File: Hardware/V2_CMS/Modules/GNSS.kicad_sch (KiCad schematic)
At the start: 20 parts, among them J3 132134, Q1 SI2302, U3 NEO-M8M, U4 AS193-73

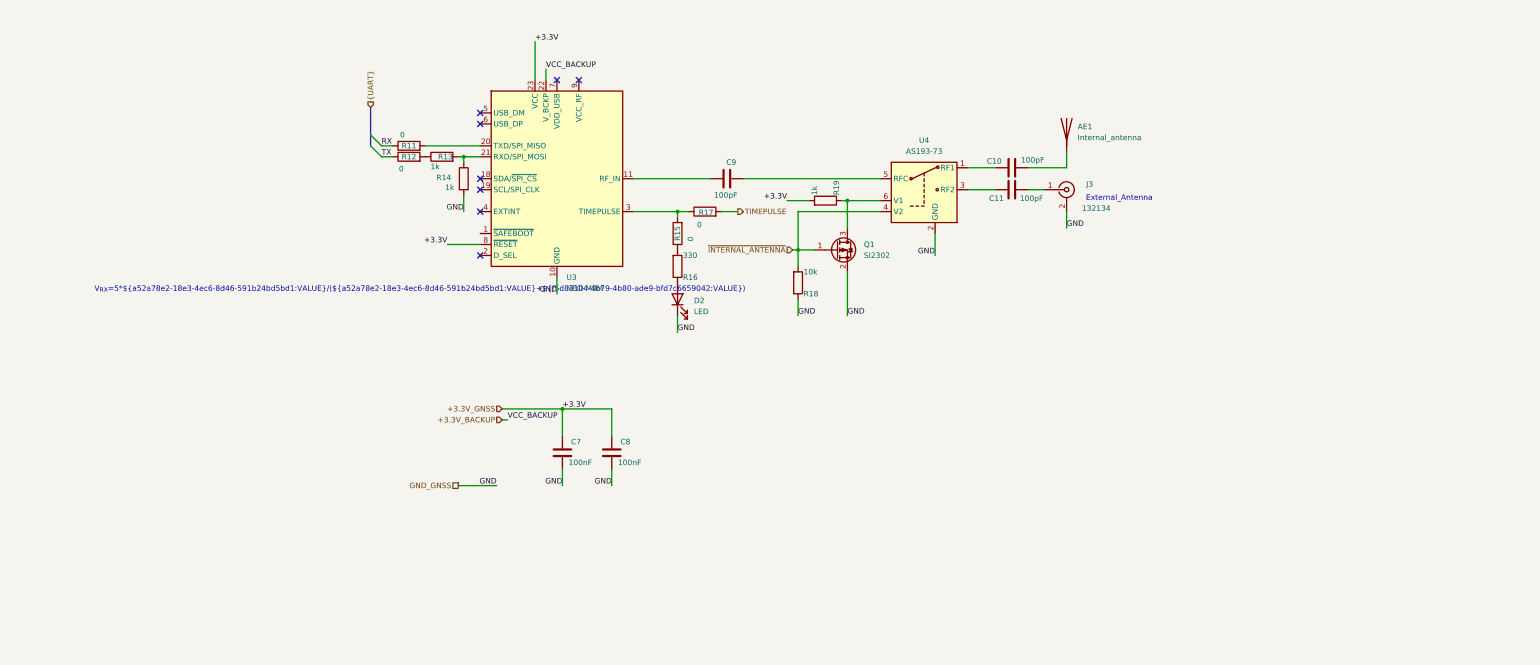
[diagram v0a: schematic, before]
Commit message: update of directory
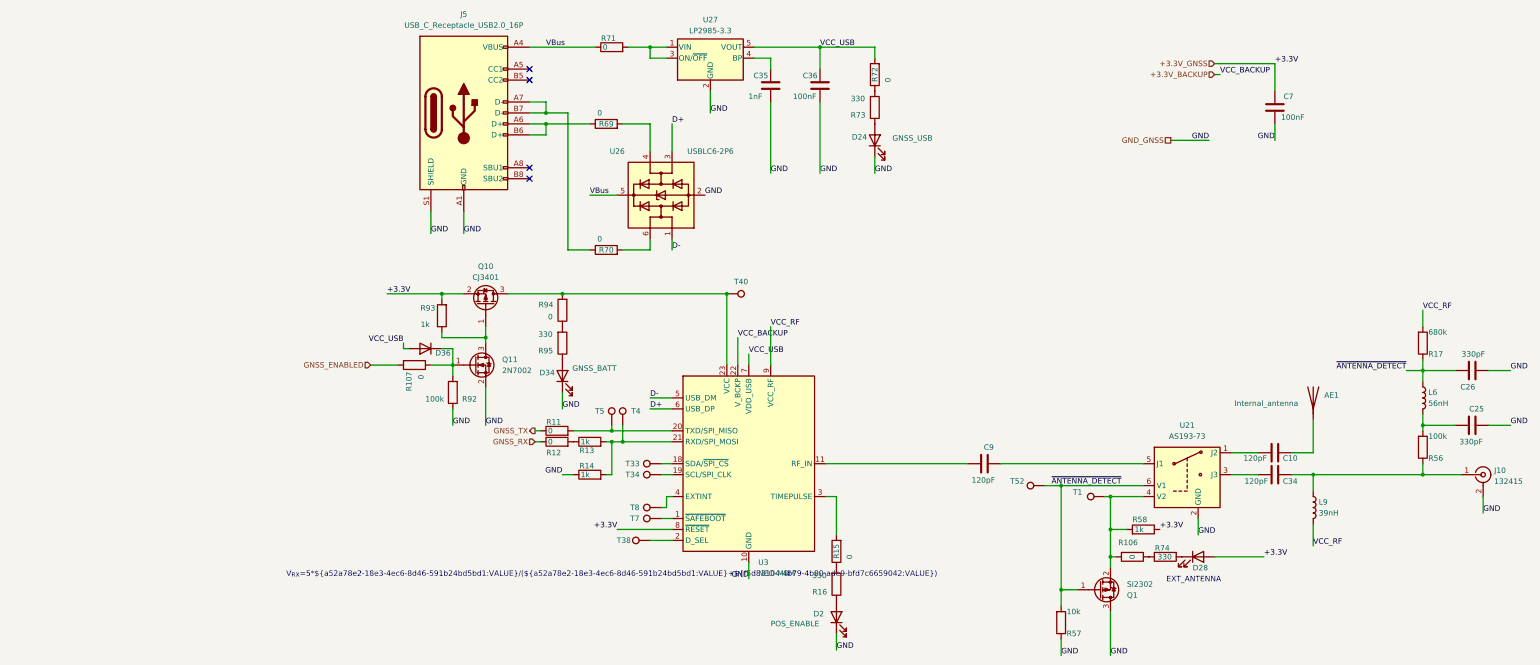
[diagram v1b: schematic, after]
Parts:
- removed C11: 100pF, Capacitor_SMD:C_0603_1608Metric, symbol Device:C
- removed C8: 100nF, Capacitor_SMD:C_0603_1608Metric, symbol Device:C
- removed J3: 132134, Connector_Coaxial:SMA_Molex_73251-1153_EdgeMount_Horizontal, symbol Connector:Conn_Coaxial
- removed R18: 10k, Resistor_SMD:R_0603_1608Metric, symbol Device:R
- removed R19: 1k, Resistor_SMD:R_0603_1608Metric, symbol Device:R
- removed U4: AS193-73, Package_TO_SOT_SMD:SOT-23-6, symbol RF_Switch:MASWSS0179
- added C25, C26: 330pF, Capacitor_SMD:C_0603_1608Metric, symbol Device:C
- added C34: 120pF, Capacitor_SMD:C_0603_1608Metric, symbol Device:C
- added C35: 1nF, Capacitor_SMD:C_0603_1608Metric, symbol Device:C
- added C36: 100nF, Capacitor_SMD:C_0603_1608Metric, symbol Device:C
- added D24: GNSS_USB, LED_SMD:LED_0603_1608Metric, symbol Device:LED
- added D28: LED_EXT_ANTENNA, LED_SMD:LED_0603_1608Metric, symbol Device:LED
- added D34: GNSS_BATT, LED_SMD:LED_0603_1608Metric, symbol Device:LED
- added D36: 1N4148, Diode_SMD:D_SOD-323, symbol Diode:1N4148
- added J10: 132415, Connector_Coaxial:SMA_Molex_73251-1153_EdgeMount_Horizontal, symbol Connector:Conn_Coaxial
- added J5: USB_C_Receptacle_USB2.0_16P, Connector_USB:USB_C_Receptacle_GCT_USB4085, symbol Connector:USB_C_Receptacle_USB2.0_16P
- added L6: 56nH, Inductor_SMD:L_0603_1608Metric, symbol Device:L
- added L9: 39nH, Inductor_SMD:L_0603_1608Metric, symbol Device:L
- added Q10: CJ3401, Package_TO_SOT_SMD:SOT-23, symbol Transistor_FET:FDN340P
- added Q11: 2N7002, Package_TO_SOT_SMD:SOT-23, symbol Transistor_FET:2N7002
- added R106, R107, R69, R70, R71, R72, R94: 0, Resistor_SMD:R_0603_1608Metric, symbol Device:R
- added R56, R92: 100k, Resistor_SMD:R_0603_1608Metric, symbol Device:R
- added R57: 10k, Resistor_SMD:R_0603_1608Metric, symbol Device:R
- added R58, R93: 1k, Resistor_SMD:R_0603_1608Metric, symbol Device:R
- added R73, R74, R95: 330, Resistor_SMD:R_0603_1608Metric, symbol Device:R
- added T1, T33, T34, T38, T4, T40, T5, T52, T7, T8: TP, TestPoint:TestPoint_Pad_D1.0mm, symbol Connector:TestPoint
- added U21: AS193-73, Package_TO_SOT_SMD:SOT-23-6, symbol RF_Switch:MASWSS0179
- added U26: USBLC6-2P6, Package_TO_SOT_SMD:SOT-666, symbol Power_Protection:USBLC6-2P6
- added U27: LP2985-3.3, Package_TO_SOT_SMD:SOT-23-5, symbol Regulator_Linear:LP2985-3.3
- C10, C9: value 100pF -> 120pF
- D2: value LED -> POS_ENABLE
- R17: value 0 -> 680k
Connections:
- net TIMEPULSE is gone; now on net VCC_RF: R17.2
- net +3.3V_GNSS: now also D28.2 (A), Q10.2 (S), R58.1, R93.2; no longer U3.23 (VCC)
- net GND_GNSS: now also Q1.3 (D), R14.1, C25.1, C26.2, C35.2, C36.2, D24.1 (K), D34.1 (K), J10.2 (Ext), J5.A1 (GND), J5.A12 (GND), J5.B1 (GND), J5.B12 (GND), J5.S1 (SHIELD), Q11.2 (S), R57.1, R92.1, U21.2 (GND), U26.2 (GND), U27.2 (GND); no longer Q1.2 (S), R14.2
- net at R15.2, U3.3 (TIMEPULSE): no longer R17.1
- net at C9.1: now also U21.5 (J1)
- net at C10.1: now also U21.1 (J2); no longer AE1.1 (A)
- net at C10.2: now also AE1.1 (A)
- net at R11.2, U3.20 (TXD/SPI_MISO): now also T5.1
- net at R13.2, U3.21 (RXD/SPI_MOSI): now also R14.2, T4.1; no longer R14.1
- net at U3.1 (~{SAFEBOOT}): now also T7.1
- net at U3.18 (SDA/~{SPI_CS}): now also T33.1
- net at U3.19 (SCL/SPI_CLK): now also T34.1
- net at U3.2 (D_SEL): now also T38.1
- net at U3.4 (EXTINT): now also T8.1
- net D-: now reaches U3.5 (USB_DM)
- net D-: now also U26.1 (I/O1)
- net D+: now reaches U3.6 (USB_DP)
- net D+: now also U26.3 (I/O2)
- net VCC_USB: now reaches U3.7 (VDD_USB)
- net VCC_USB: now also C36.1, D36.2 (A), R72.2, U27.5 (VOUT)
- net VCC_RF: now reaches U3.9 (VCC_RF)
- net VCC_RF: now also L9.2
- net RX renamed GNSS_TX
- net TX renamed GNSS_RX
- net ~{INTERNAL_ANTENNA} renamed ~{ANTENNA_DETECT}
- net ~{ANTENNA_DETECT}: now also R17.1, C26.1, L6.1, R57.2, T52.1, U21.6 (V1)
- new net: D24.2 (A), R73.1
- new net: C34.2, J10.1 (In), L9.1, R56.1
- new net: D36.1 (K), Q11.1 (G), R107.1, R92.2
- new net: Q1.2 (S), R106.2, R58.2, T1.1, U21.4 (V2)
- new net: R106.1, R74.1
- new net: D28.1 (K), R74.2
- new net: J5.A6 (D+), J5.B6 (D+), R69.1
- new net: R69.2, U26.4 (I/O2)
- new net: R72.1, R73.2
- new net: Q10.1 (G), Q11.3 (D), R93.1
- new net: Q10.3 (D), R94.2, T40.1, U3.23 (VCC)
- new net: C25.2, L6.2, R56.2
- new net: R94.1, R95.2
- new net: J5.A7 (D-), J5.B7 (D-), R70.1
- new net: C34.1, U21.3 (J3)
- new net: D34.2 (A), R95.1
- new net: R70.2, U26.6 (I/O1)
- new net: C35.1, U27.4 (BP)
- new net: R71.2, U27.1 (VIN), U27.3 (ON/~{OFF})
- new net GNSS_ENABLED: R107.2
- new net VBus: J5.A4 (VBUS), J5.A9 (VBUS), J5.B4 (VBUS), J5.B9 (VBUS), R71.1, U26.5 (VBUS)
- no-connect marks 8 -> 4
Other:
- note added: "EXT_ANTENNA"
- note removed: "External_Antenna"
- moved on the sheet: AE1, C7, C9, D2, R11, R12, R13, R14, R15, R16, U3
